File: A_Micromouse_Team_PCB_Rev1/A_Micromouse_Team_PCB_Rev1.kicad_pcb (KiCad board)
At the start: 2 copper layers, 45.5 x 48 mm, 23 parts, among them J1 TOF2, J10 5V->12V, J11 MotorCageMount, J12 MotorCageMount, J2 TOF3, J3 TOF4, J4 TOF5, J5 Motor1, J6 Motor2, J7 NeoPixel, J8 TOF1, J9 Battery, SW1 SW_DIP_x06, U1 Teensy4.0, U2 IMU, U3 MotorController

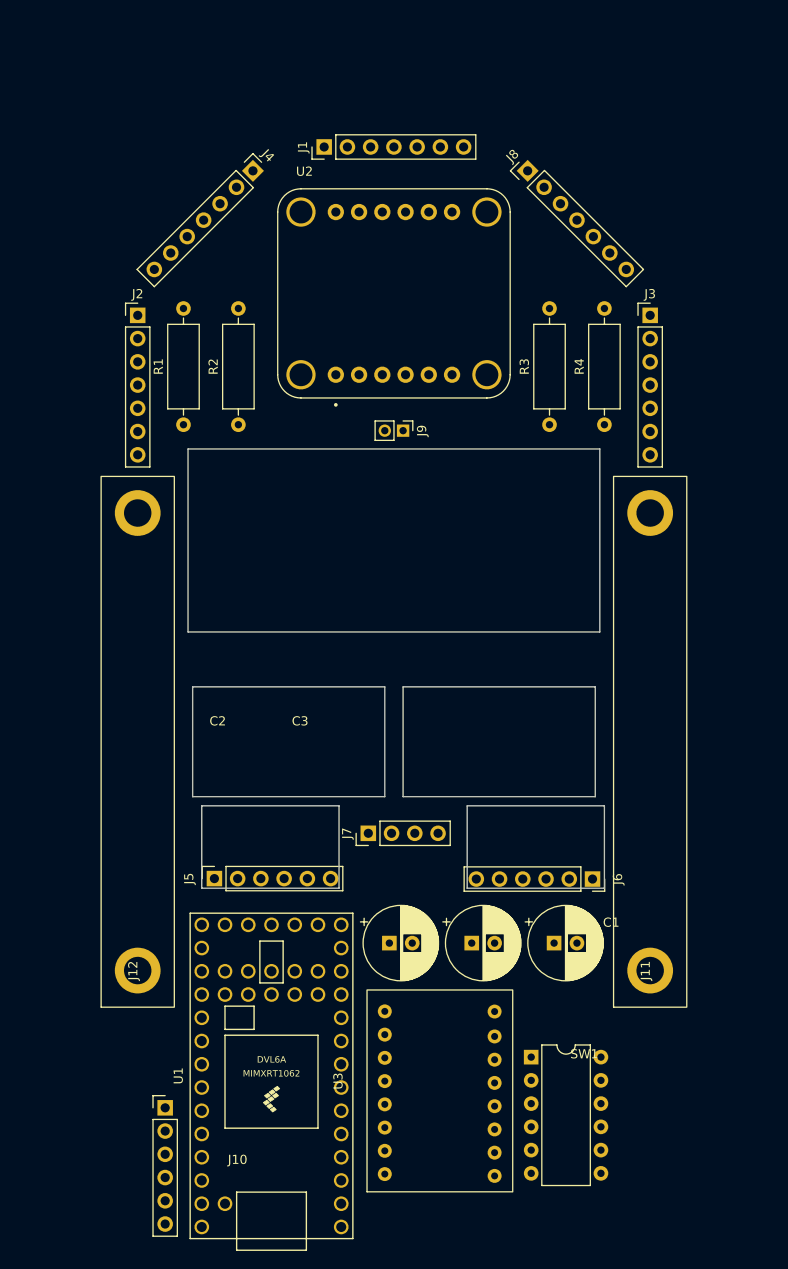
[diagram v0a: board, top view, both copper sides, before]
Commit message: Add files via upload
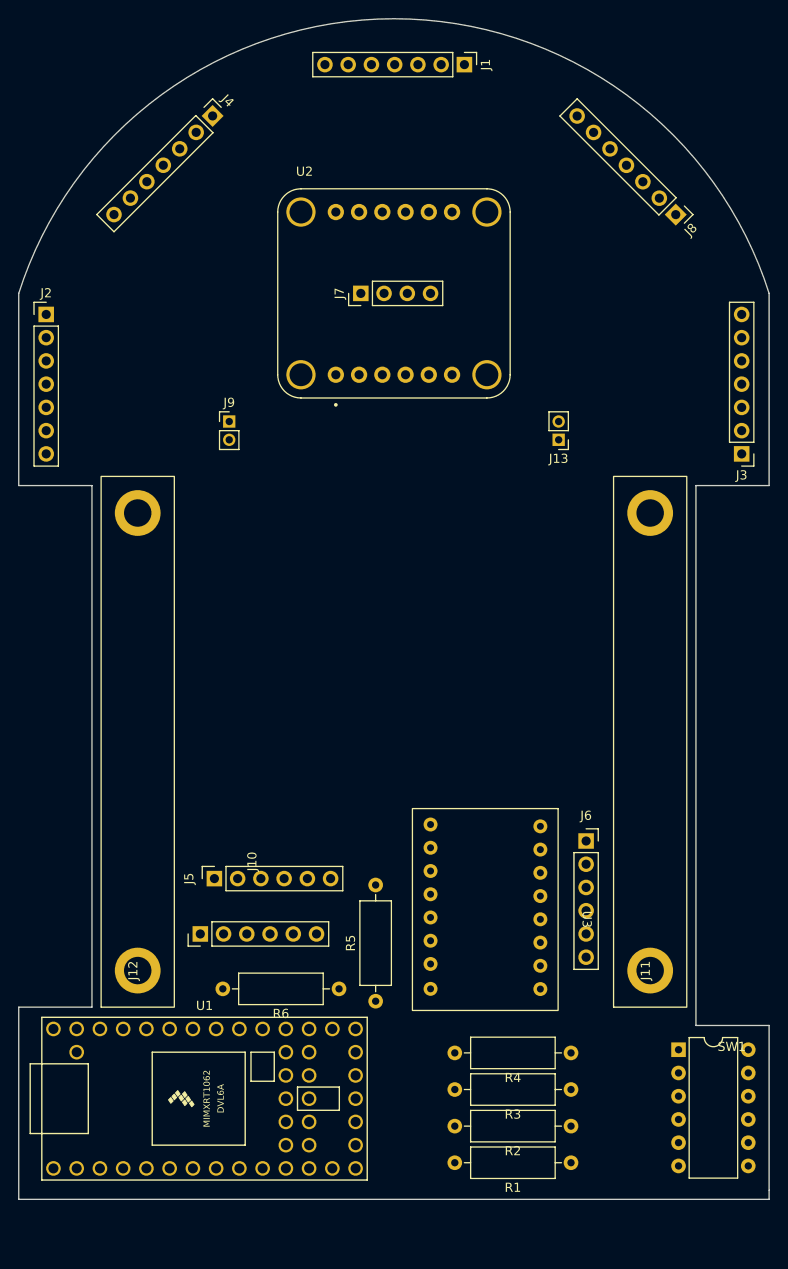
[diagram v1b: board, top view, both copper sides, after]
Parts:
- removed C1, C2, C3: C, Capacitor_THT:CP_Radial_D8.0mm_P2.50mm
- added J13: Battery, Connector_PinHeader_2.00mm:PinHeader_1x02_P2.00mm_Vertical, F.Cu at (163.0, 91.0)
- added R5: R_US, Resistor_THT:R_Axial_DIN0309_L9.0mm_D3.2mm_P12.70mm_Horizontal, F.Cu at (143.0, 152.3)
- added R6: R_US, Resistor_THT:R_Axial_DIN0309_L9.0mm_D3.2mm_P12.70mm_Horizontal, F.Cu at (139.0, 151.0)
- J2: value TOF3 -> locked
- moved R1 91.1 mm to (164.3, 170.0), turned to 180 degrees
- moved R2 84.8 mm to (164.3, 166.0), turned to 180 degrees
- moved R3 72.7 mm to (164.3, 162.0), turned to 180 degrees
- moved R4 68.7 mm to (164.3, 158.0), turned to 180 degrees
- moved J7 59.0 mm to (141.4, 75.0)
- moved U3 41.6 mm to (161.0, 133.2), turned to -90 degrees
- moved J10 19.4 mm to (123.8, 145.0), turned to 90 degrees
- moved J9 19.0 mm to (127.0, 89.0), turned to 0 degrees
- moved J3 18.1 mm to (183.0, 92.5), turned to 180 degrees
- moved J1 17.8 mm to (152.7, 50.0), turned to -90 degrees
- moved J8 16.9 mm to (175.8, 66.4), turned to -135 degrees
- moved SW1 16.1 mm to (176.1, 157.7)
- moved J2 10.0 mm to (107.0, 77.3)
- moved U1 7.73 mm to (124.3, 163.0), turned to 0 degrees
- moved J4 7.45 mm to (125.2, 55.6)
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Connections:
- J10 pad 4: +5V -> +5VD
- J10 pad 5: unconnected-(J10-Pin_5-Pad5) -> +5VD
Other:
- board size 45.5 x 48 mm -> 82 x 129 mm
